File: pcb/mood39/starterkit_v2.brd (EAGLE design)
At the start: 32 x 32 mm, 19 parts, among them IC1 TINY85, IC2 LP2950

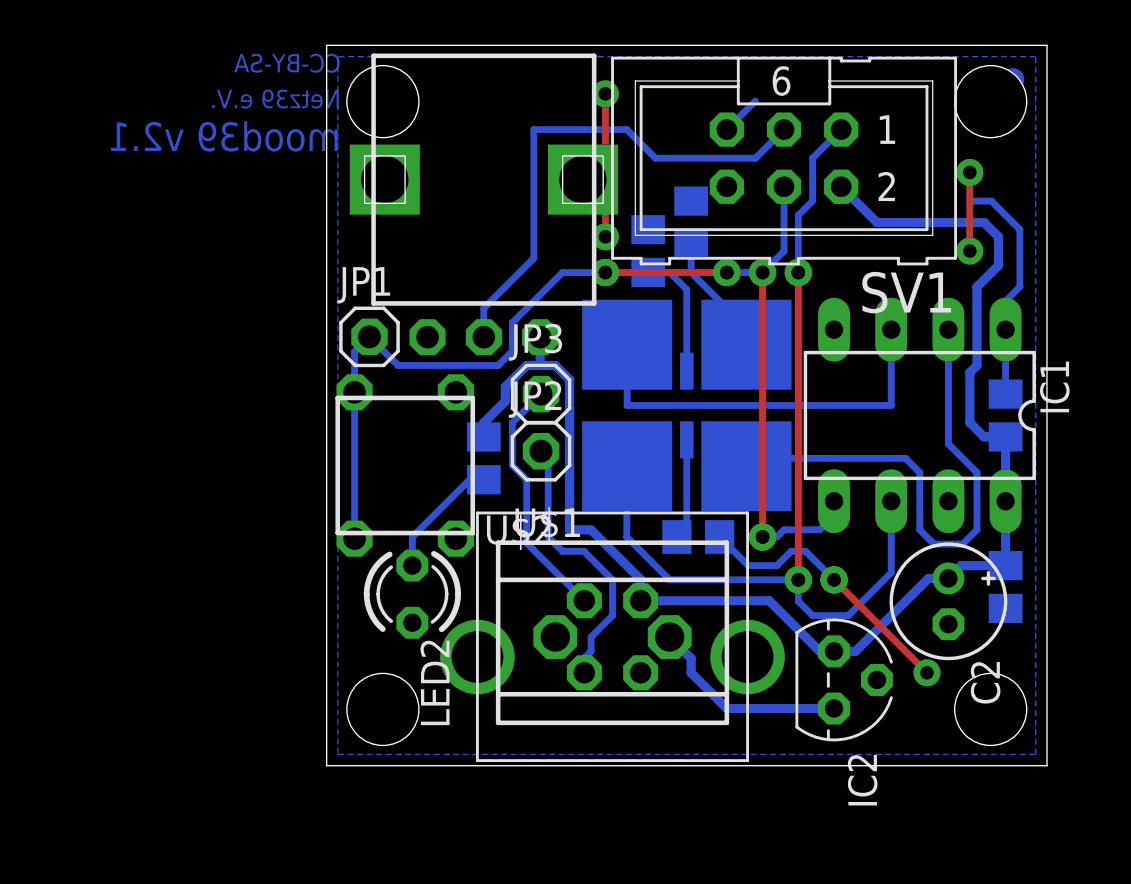
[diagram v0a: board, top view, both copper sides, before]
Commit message: no real improvement, this seemed more promising
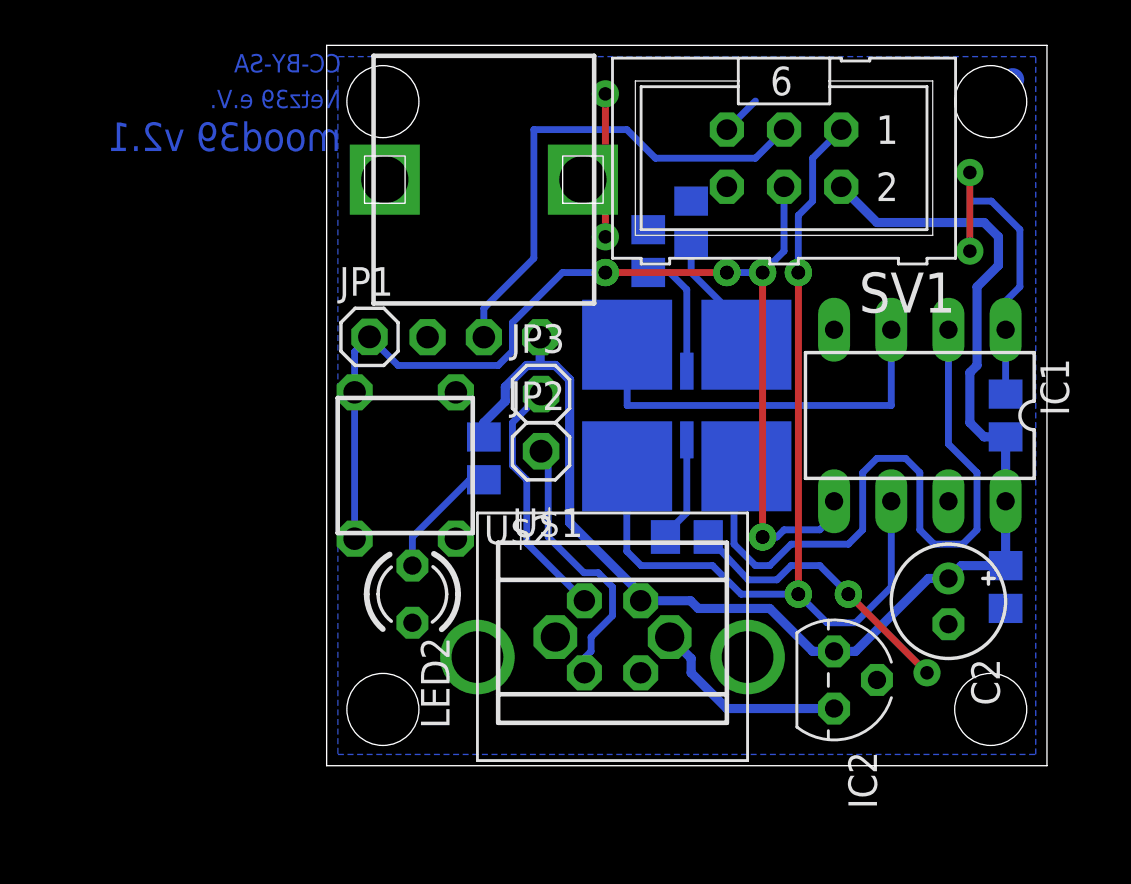
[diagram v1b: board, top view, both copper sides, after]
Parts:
- moved R3 0.51 mm to (16.0, 10.2)
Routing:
- net PB3: track 23.1 -> 31.1 mm
- net MISO: track 41.7 -> 42.7 mm
- net VCC: track 62.1 -> 61.5 mm
- net GND: track 22.1 -> 22.6 mm
